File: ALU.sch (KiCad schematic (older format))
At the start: 30 parts, among them U44 74LS245, U45 74LS00, U46 74LS86, U47 74LS86, U48 74LS86, U49 74LS00, U50 74LS86, U51 74HC02, U52 74LS00, U53 74LS00, U54 74LS283, U55 74LS85, U56 74LS283, U57 74LS245, U58 74LS85, U59 74LS245, U60 74LS283, U61 74LS85, U62 74LS173, U63 74LS283, U64 74LS245, U65 74LS85

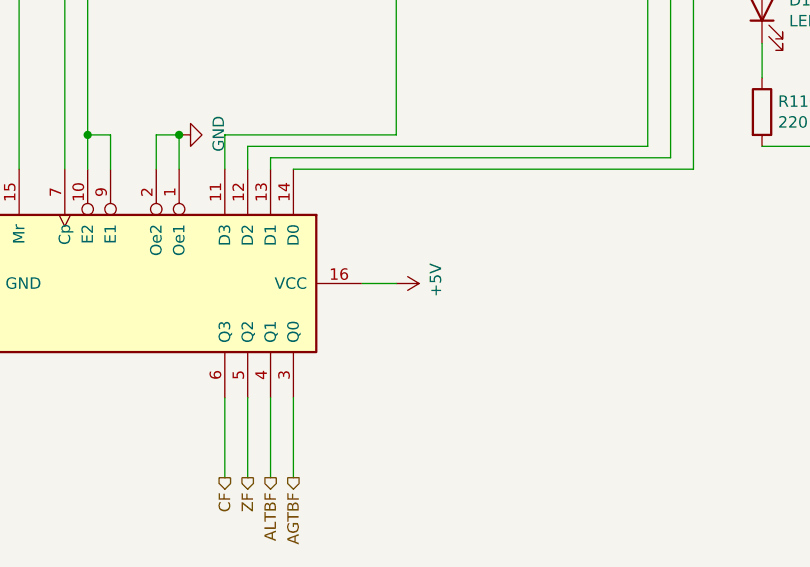
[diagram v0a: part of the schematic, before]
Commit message: fixed more errors
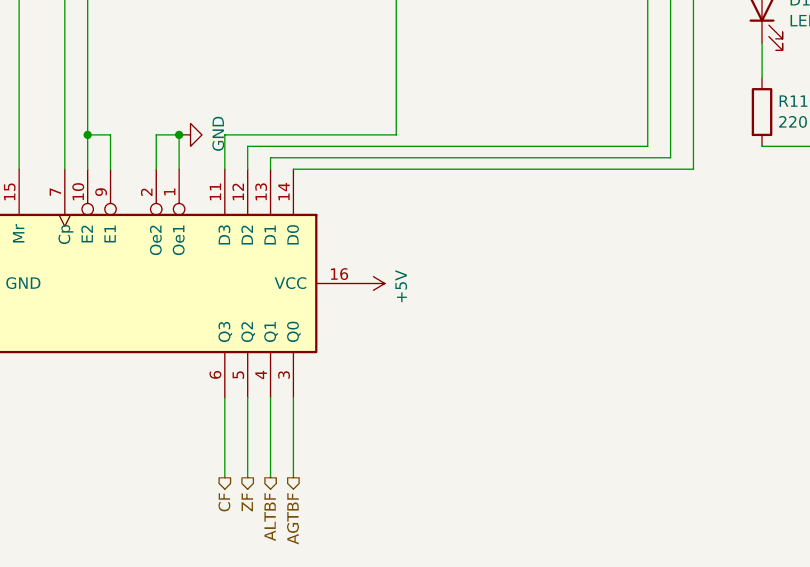
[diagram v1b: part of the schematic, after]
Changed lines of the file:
@@
-$EndComp
-$Comp
-L 16bitCpu-rescue:+5V-power #PWR?
-U 1 1 60667C5F
-P 14100 17800
-AR Path="/60667C5F" Ref="#PWR?"  Part="1"
-AR Path="/5F5F4A69/60667C5F" Ref="#PWR0177"  Part="1"
-F 0 "#PWR0177" H 14100 17650 50  0001 C CNN
-F 1 "+5V" H 14115 17973 50  0000 C CNN
-F 2 "" H 14100 17800 50  0001 C CNN
-F 3 "" H 14100 17800 50  0001 C CNN
-	1    14100 17800
-	0    -1   -1   0
 $EndComp
 $Comp
@@
 Wire Wire Line
 	5350 18650 4900 18650
-$Comp
-L 16bitCpu-rescue:+5V-power #PWR0188
-U 1 1 5F826AFE
-P 18350 17850
-F 0 "#PWR0188" H 18350 17700 50  0001 C CNN
-F 1 "+5V" H 18365 18023 50  0000 C CNN
-F 2 "" H 18350 17850 50  0001 C CNN
-F 3 "" H 18350 17850 50  0001 C CNN
-	1    18350 17850
-	0    1    -1   0
-$EndComp
-Wire Wire Line
-	18200 17850 18350 17850
 Text HLabel 17700 18700 3    50   Output ~ 0
 ZF
@@
 	7050 10650 8600 10650
 Connection ~ 10450 4900
+$Comp
+L 16bitCpu-rescue:+5V-power #PWR?
+U 1 1 63E4B52F
+P 18200 17850
+AR Path="/63E4B52F" Ref="#PWR?"  Part="1"
+AR Path="/5F5F4A69/63E4B52F" Ref="#PWR0136"  Part="1"
+F 0 "#PWR0136" H 18200 17700 50  0001 C CNN
+F 1 "+5V" H 18215 18023 50  0000 C CNN
+F 2 "" H 18200 17850 50  0001 C CNN
+F 3 "" H 18200 17850 50  0001 C CNN
+	1    18200 17850
+	0    1    1    0
+$EndComp
+$Comp
+L 16bitCpu-rescue:+5V-power #PWR?
+U 1 1 63F666EC
+P 14100 17800
+AR Path="/63F666EC" Ref="#PWR?"  Part="1"
+AR Path="/5F5F4A69/63F666EC" Ref="#PWR0177"  Part="1"
+F 0 "#PWR0177" H 14100 17650 50  0001 C CNN
+F 1 "+5V" H 14115 17973 50  0000 C CNN
+F 2 "" H 14100 17800 50  0001 C CNN
+F 3 "" H 14100 17800 50  0001 C CNN
+	1    14100 17800
+	0    -1   -1   0
+$EndComp
 $EndSCHEMATC
